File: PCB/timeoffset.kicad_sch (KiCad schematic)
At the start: 11 parts, among them J1 Conn_01x03, J2 Conn_01x03, Q1 IRF7204_jandevalua, U1 ATtiny13A-SU

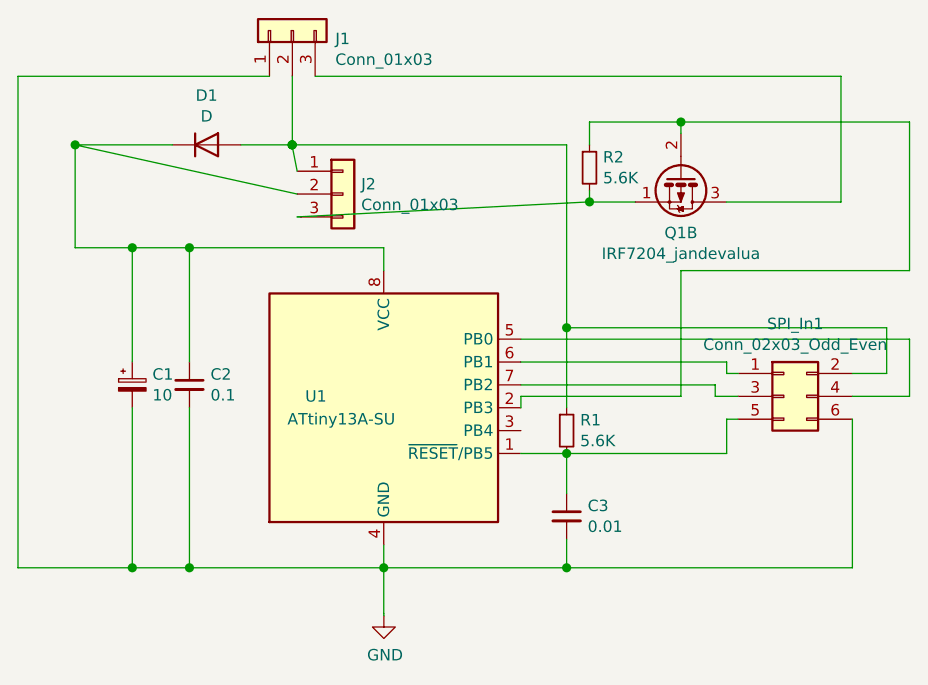
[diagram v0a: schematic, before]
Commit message: board optimization
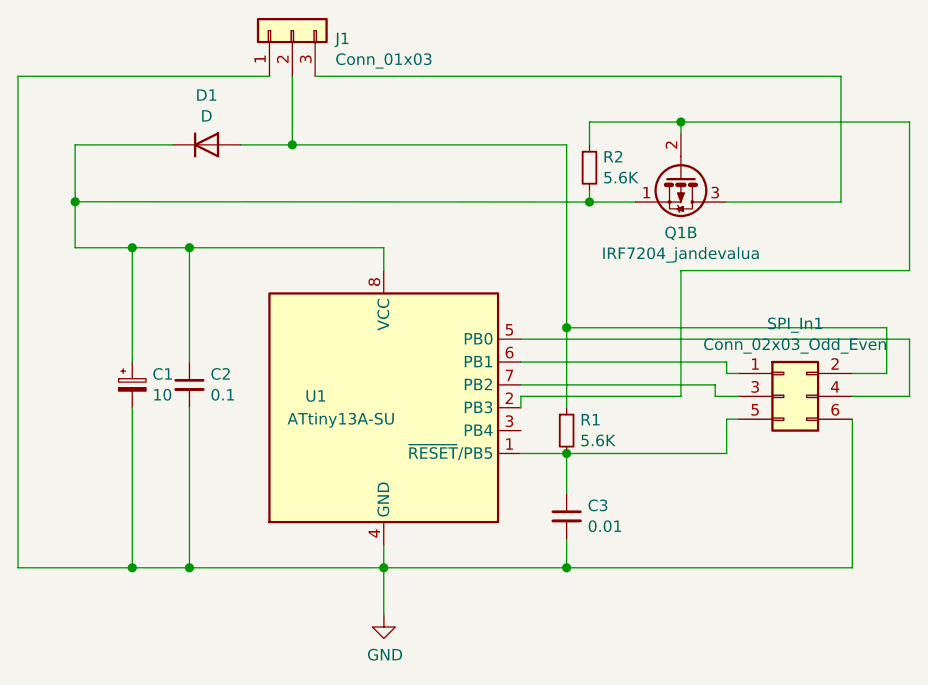
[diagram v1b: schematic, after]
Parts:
- removed J2: Conn_01x03, Connector_JST:JST_PH_S3B-PH-K_1x03_P2.00mm_Horizontal, symbol Connector_Generic:Conn_01x03
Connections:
- net at C1.1, C2.1, D1.1 (K)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: now also Q1.1 (S2), R2.2
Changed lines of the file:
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@@
 (kicad_sch (version 20210621) (generator eeschema)
   (paper "A4")
-  (junction (at 64.77 40.64) (diameter 1.016) (color 0 0 0 0))
+  (junction (at 64.77 46.961) (diameter 1.016) (color 0 0 0 0))
   (junction (at 71.12 52.07) (diameter 1.016) (color 0 0 0 0))
   (junction (at 71.12 87.63) (diameter 1.016) (color 0 0 0 0))
   (junction (at 77.47 52.07) (diameter 1.016) (color 0 0 0 0))
   (junction (at 77.47 87.63) (diameter 1.016) (color 0 0 0 0))
-  (junction (at 88.8615 40.64) (diameter 1.016) (color 0 0 0 0))
   (junction (at 88.9 40.64) (diameter 1.016) (color 0 0 0 0))
   (junction (at 99.06 87.63) (diameter 1.016) (color 0 0 0 0))
@@
   (junction (at 119.38 74.93) (diameter 1.016) (color 0 0 0 0))
   (junction (at 119.38 87.63) (diameter 1.016) (color 0 0 0 0))
-  (junction (at 121.92 46.9746) (diameter 1.016) (color 0 0 0 0))
+  (junction (at 121.92 46.99) (diameter 1.016) (color 0 0 0 0))
   (junction (at 132.08 38.1) (diameter 1.016) (color 0 0 0 0))
   (wire (pts (xy 58.42 33.02) (xy 58.42 87.63))
@@
     (stroke (width 0) (type solid) (color 0 0 0 0))
   )
-  (wire (pts (xy 64.77 40.64) (xy 64.77 52.07))
+  (wire (pts (xy 64.77 40.64) (xy 64.77 46.961))
+    (stroke (width 0) (type solid) (color 0 0 0 0))
+  )
+  (wire (pts (xy 64.77 46.961) (xy 64.77 52.07))
     (stroke (width 0) (type solid) (color 0 0 0 0))
   )
@@
     (stroke (width 0) (type solid) (color 0 0 0 0))
   )
-  (wire (pts (xy 88.8615 40.64) (xy 83.185 40.64))
+  (wire (pts (xy 83.185 40.64) (xy 88.9 40.64))
     (stroke (width 0) (type solid) (color 0 0 0 0))
   )
@@
     (stroke (width 0) (type solid) (color 0 0 0 0))
   )
-  (wire (pts (xy 88.9 40.64) (xy 88.8615 40.64))
-    (stroke (width 0) (type solid) (color 0 0 0 0))
-  )
-  (wire (pts (xy 89.4385 43.5642) (xy 88.8615 40.64))
-    (stroke (width 0) (type solid) (color 0 0 0 0))
-  )
-  (wire (pts (xy 89.4385 46.1042) (xy 64.77 40.64))
-    (stroke (width 0) (type solid) (color 0 0 0 0))
-  )
-  (wire (pts (xy 89.4385 48.6442) (xy 121.92 46.9746))
-    (stroke (width 0) (type solid) (color 0 0 0 0))
-  )
   (wire (pts (xy 99.06 52.07) (xy 77.47 52.07))
     (stroke (width 0) (type solid) (color 0 0 0 0))
@@
     (stroke (width 0) (type solid) (color 0 0 0 0))
   )
-  (wire (pts (xy 121.92 45.72) (xy 121.92 46.9746))
-    (stroke (width 0) (type solid) (color 0 0 0 0))
-  )
-  (wire (pts (xy 121.92 46.9746) (xy 121.92 46.99))
+  (wire (pts (xy 121.92 45.72) (xy 121.92 46.99))
+    (stroke (width 0) (type solid) (color 0 0 0 0))
+  )
+  (wire (pts (xy 121.92 46.99) (xy 64.77 46.961))
     (stroke (width 0) (type solid) (color 0 0 0 0))
   )
@@
     )
     (property "Datasheet" "~" (id 3) (at 88.9 27.94 0)
-      (effects (font (size 1.27 1.27)) hide)
-    )
-    (pin "1")
-    (pin "2")
-    (pin "3")
-  )
-  (symbol (lib_id "Connector_Generic:Conn_01x03") (at 94.5185 46.1042 0) (unit 1)
-    (in_bom yes) (on_board yes)
-    (property "Reference" "J2" (id 0) (at 96.5506 45.0056 0)
-      (effects (font (size 1.27 1.27)) (justify left))
-    )
-    (property "Value" "Conn_01x03" (id 1) (at 96.5506 47.3043 0)
-      (effects (font (size 1.27 1.27)) (justify left))
-    )
-    (property "Footprint" "Connector_JST:JST_PH_S3B-PH-K_1x03_P2.00mm_Horizontal" (id 2) (at 94.5185 46.1042 0)
-      (effects (font (size 1.27 1.27)) hide)
-    )
-    (property "Datasheet" "~" (id 3) (at 94.5185 46.1042 0)
       (effects (font (size 1.27 1.27)) hide)
     )
@@
       (reference "J1") (unit 1) (value "Conn_01x03") (footprint "Connector_PinHeader_2.54mm:PinHeader_1x03_P2.54mm_Vertical")
     )
-    (path "/33fe6c4e-0011-4e87-b903-abc10fce3756"
-      (reference "J2") (unit 1) (value "Conn_01x03") (footprint "Connector_JST:JST_PH_S3B-PH-K_1x03_P2.00mm_Horizontal")
-    )
     (path "/00000000-0000-0000-0000-00005de29fca"
